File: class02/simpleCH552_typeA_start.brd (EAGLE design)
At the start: 40.6 x 12 mm, 9 parts, among them U2 CH552G, X1 USBPCB

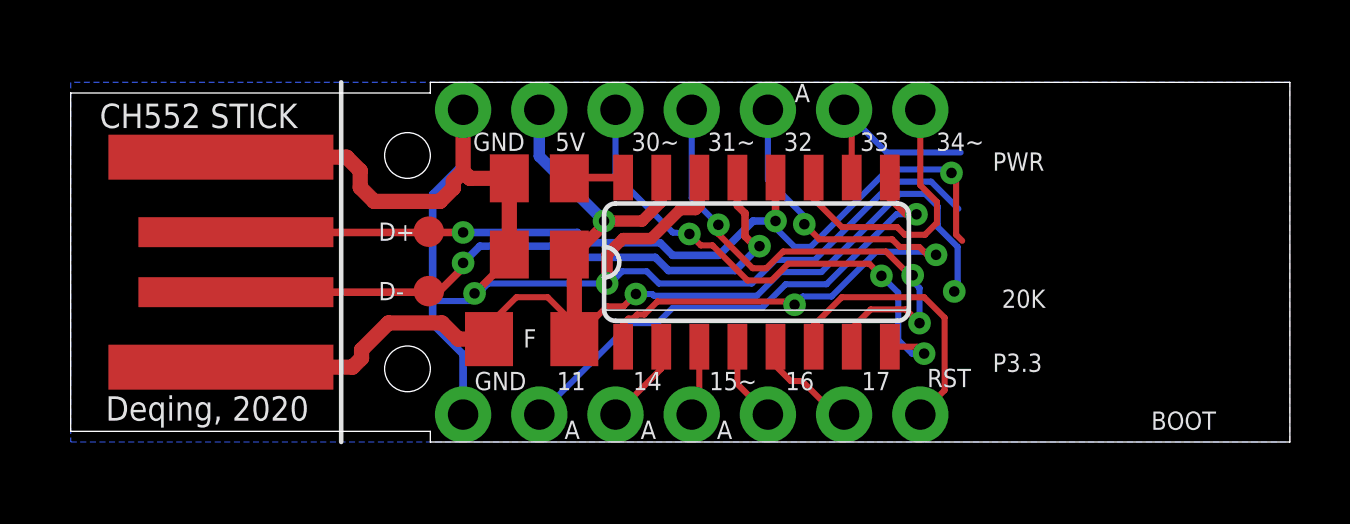
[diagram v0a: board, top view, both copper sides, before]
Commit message: change start
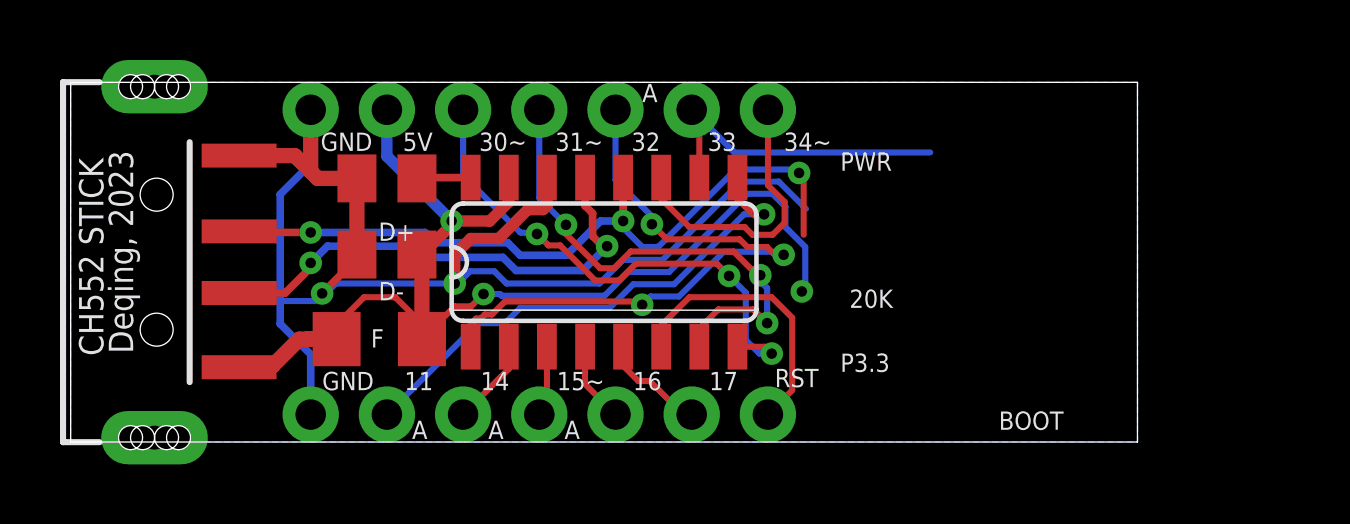
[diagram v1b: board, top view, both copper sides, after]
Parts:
- removed TP1, TP2: TEST-POINT3X4, SparkFun-Connectors:PAD.03X.04
- removed X1: USBPCB, SparkFun:USB-A-PCB
- added J4: USB_A_SMT_MALE, SparkFun-Connectors:USB-A-SMT-MALE
- moved C1 5.08 mm to (10.5, 6.25)
- moved C2 5.08 mm to (10.5, 8.79)
- moved F1 5.08 mm to (10.3, 3.43)
- moved J1 5.08 mm to (8.00, 0.91)
- moved J2 5.08 mm to (8.00, 11.1)
- moved U2 5.08 mm to (17.8, 5.99)
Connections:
- net +5V: now also J4.VBUS1; no longer X1.5V
- net GND: now also J4.GND1; no longer X1.GND
- net USB_D+: now also J4.D+1; no longer TP2.P$1, X1.USB_P
- net USB_D-: now also J4.D-1; no longer TP1.P$1, X1.USB_M
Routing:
- net GND: track 54.1 -> 47.2 mm
- net USB_D+: track 31.3 -> 24.7 mm
- net USB_D-: track 21.9 -> 16.4 mm
- net +5V: track 43.8 -> 38.6 mm
- net P3.3: track 6.84 -> 10.9 mm
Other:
- board size 40.6 x 12 mm -> 35.6 x 12 mm
- board text added: "Deqing Sun 2023"
- board text added: "Deqing Sun, 2023 Prototyping Electronic Devices"
- board text added: "Deqing, 2023"
- board text added: "Try Ch55xduino with this board"
- board text removed: "Deqing Sun, 2020 Try Ch55xduino with this board"
- board text removed: "Deqing Sun, 2022 Prototyping Electronic Devices"
- board text removed: "Deqing, 2020"
